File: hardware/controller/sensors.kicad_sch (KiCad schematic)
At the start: 10 parts, among them J4 Conn_01x07, U7 MPU-6050

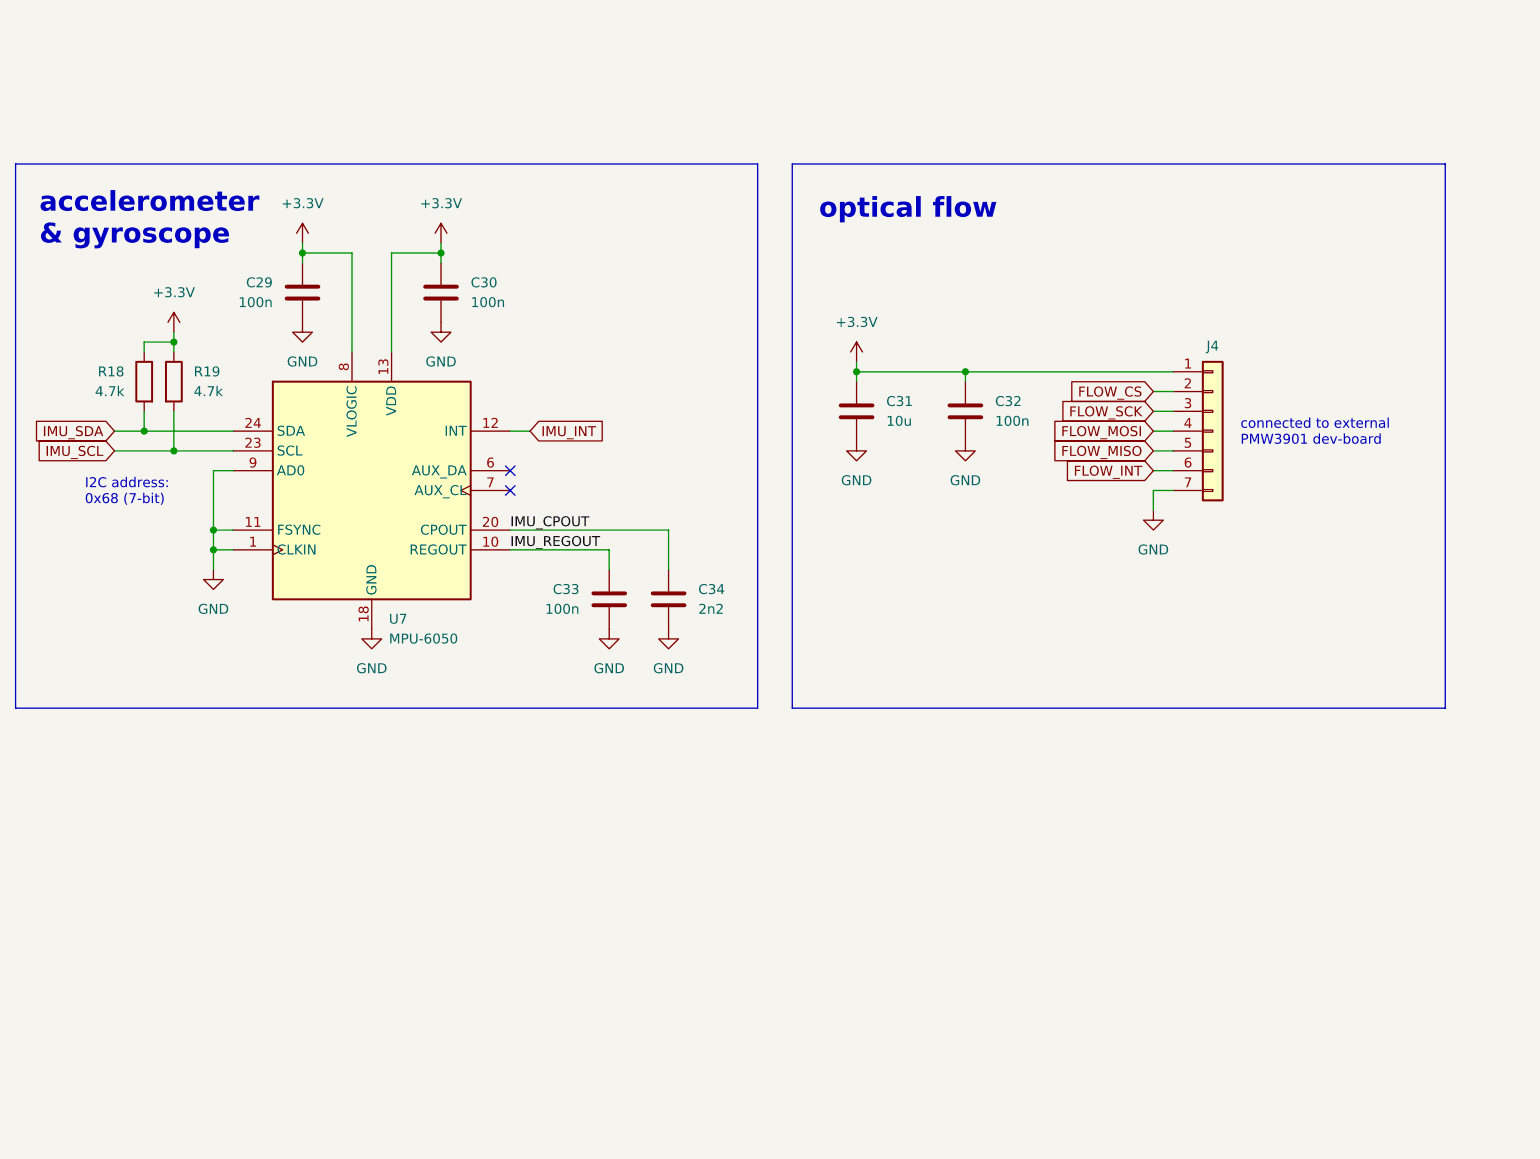
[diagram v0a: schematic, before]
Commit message: wip
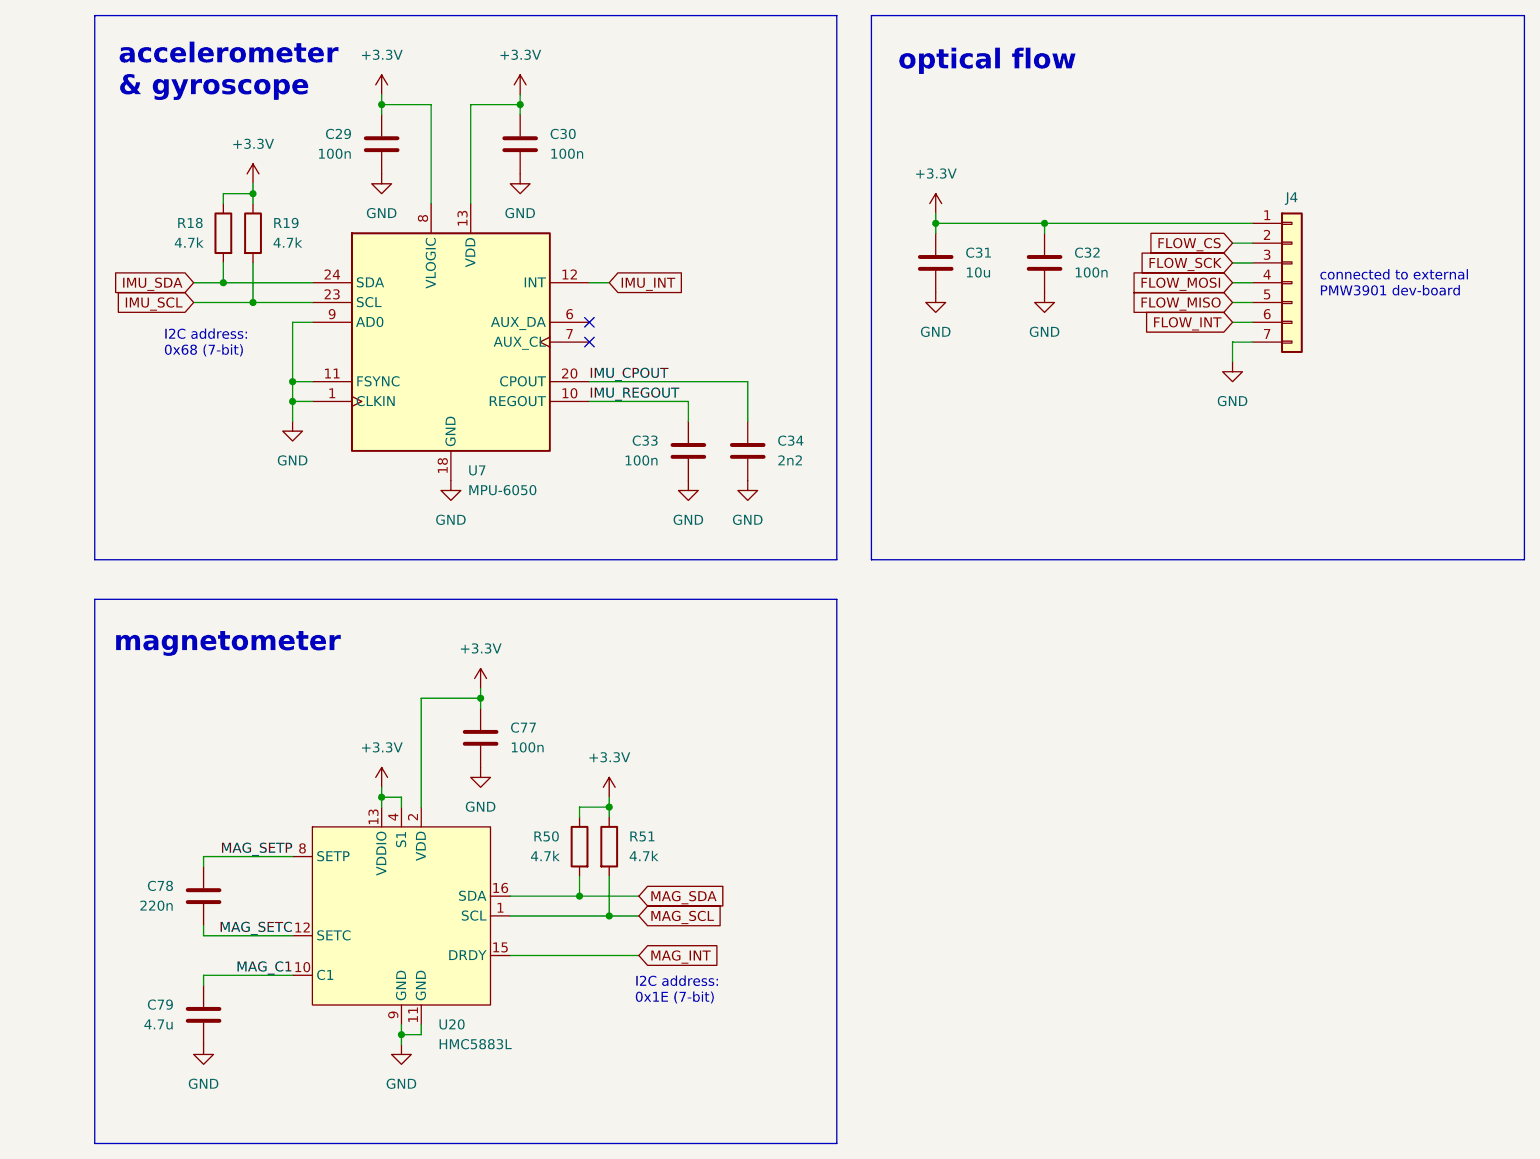
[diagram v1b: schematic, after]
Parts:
- added C77: 100n, Capacitor_SMD:C_0603_1608Metric, symbol Device:C
- added C78: 220n, Capacitor_SMD:C_0603_1608Metric, symbol Device:C
- added C79: 4.7u, Capacitor_SMD:C_0603_1608Metric, symbol Device:C
- added R50, R51: 4.7k, Resistor_SMD:R_0603_1608Metric, symbol Device:R
- added U20: HMC5883L, hogger2:HMC5883L_handsolder, symbol hogger2:HMC5883L
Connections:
- net +3.3V: now also C77.1, R50.1, R51.1, U20.13 (VDDIO), U20.2 (VDD), U20.4 (S1)
- net GND: now also C77.2, C79.2, U20.11 (GND), U20.9 (GND)
- new net MAG_C1: C79.1, U20.10 (C1)
- new net MAG_INT: U20.15 (DRDY)
- new net MAG_SCL: R51.2, U20.1 (SCL)
- new net MAG_SDA: R50.2, U20.16 (SDA)
- new net MAG_SETC: C78.2, U20.12 (SETC)
- new net MAG_SETP: C78.1, U20.8 (SETP)
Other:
- note added: "I2C address: 0x1E (7-bit)"
- note added: "magnetometer"
- moved on the sheet: C29, C30, C31, C32, C33, C34, J4, R18, R19, U7
